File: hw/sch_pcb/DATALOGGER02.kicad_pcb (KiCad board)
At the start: 2 copper layers, 80.8 x 101.1 mm, 90 parts, among them J1 HEADER_2x01_PARALLEL, J10 HEADER_2x03_PARALLEL, J11 HEADER_2x01, J12 HEADER_2x01_PARALLEL, J13 HEADER_2x01_PARALLEL, J14 HEADER_2x01_PARALLEL, J15 HEADER_2x01_PARALLEL, J16 HEADER_2x01_PARALLEL, J17 HEADER_2x01_PARALLEL, J18 HEADER_2x01_PARALLEL, J19 HEADER_2x01_PARALLEL, J2 HEADER_2x01_PARALLEL, J20 HEADER_2x01_PARALLEL, J21 HEADER_2x01, J22 HEADER_2x01_PARALLEL, J23 HEADER_2x01_PARALLEL, J24 HEADER_2x01_PARALLEL, J25 HEADER_2x01_PARALLEL, J26 HEADER_2x01_PARALLEL, J27 HEADER_2x01_PARALLEL, J28 HEADER_2x01_PARALLEL, J29 HEADER_2x01_PARALLEL, J3 HEADER_2x01_PARALLEL, J30 HEADER_2x01_PARALLEL, J31 HEADER_2x03, J32 HEADER_2x01, J33 HEADER_2x03_PARALLEL, J34 MCC-SD (kouka z modulu), J4 HEADER_2x01_PARALLEL, J5 HEADER_2x01_PARALLEL, J6 HEADER_2x03_PARALLEL, J7 MCC-SD, J8 HEADER_2x01_PARALLEL, J9 HEADER_2x01, M2 HOLE, M3 HOLE, M4 HOLE, SW1 5MS1S102AM6QE, U1 ISL21080CIH320Z-TK, U2 TPS22965-Q1, U3 ATMEGA1284P-AU, U4 PCF85263A, U5 LM4041CIM3-1.2(neosazovat), U6 AT24CS64-SSHM, Y1 16MHz, Y2 ABS07-120-32.768KHZ-T

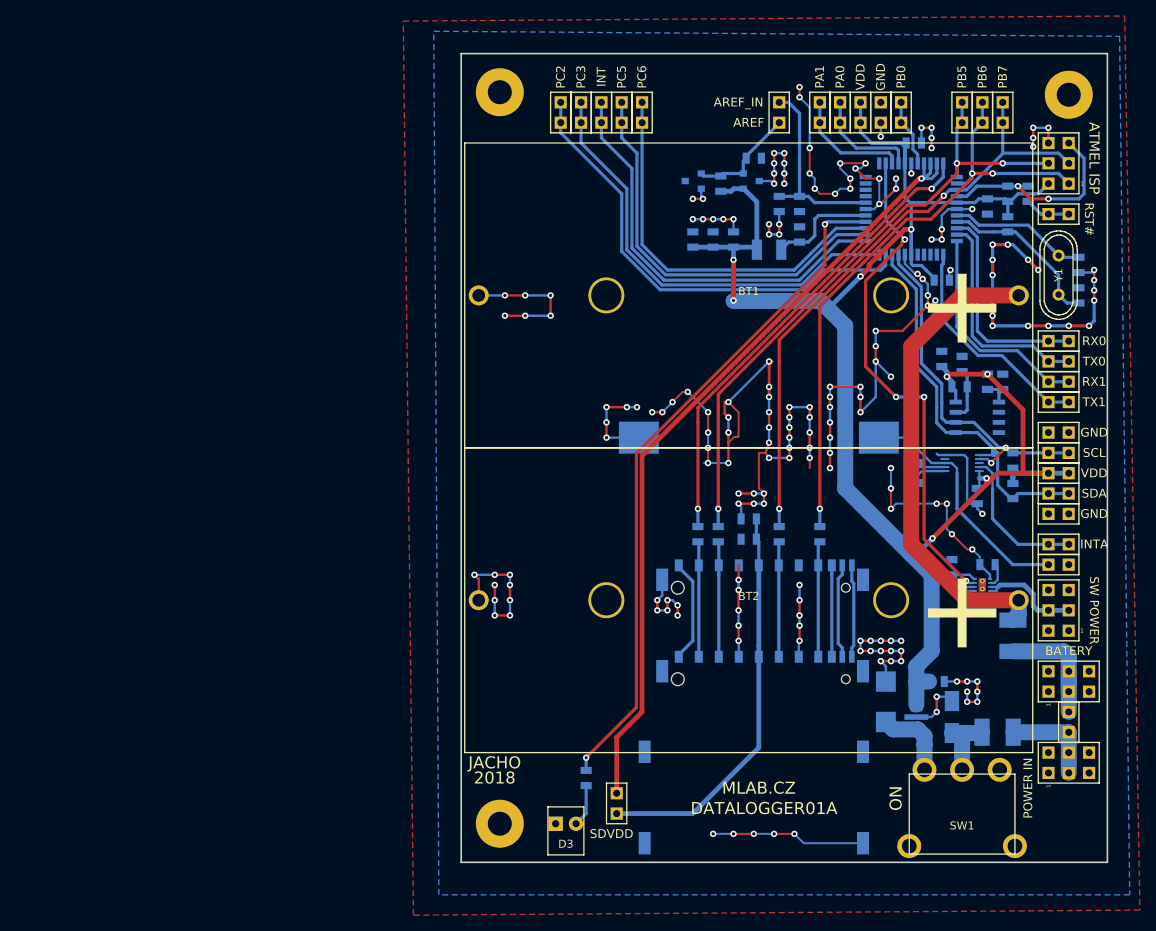
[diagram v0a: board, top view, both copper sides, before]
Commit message: progress?
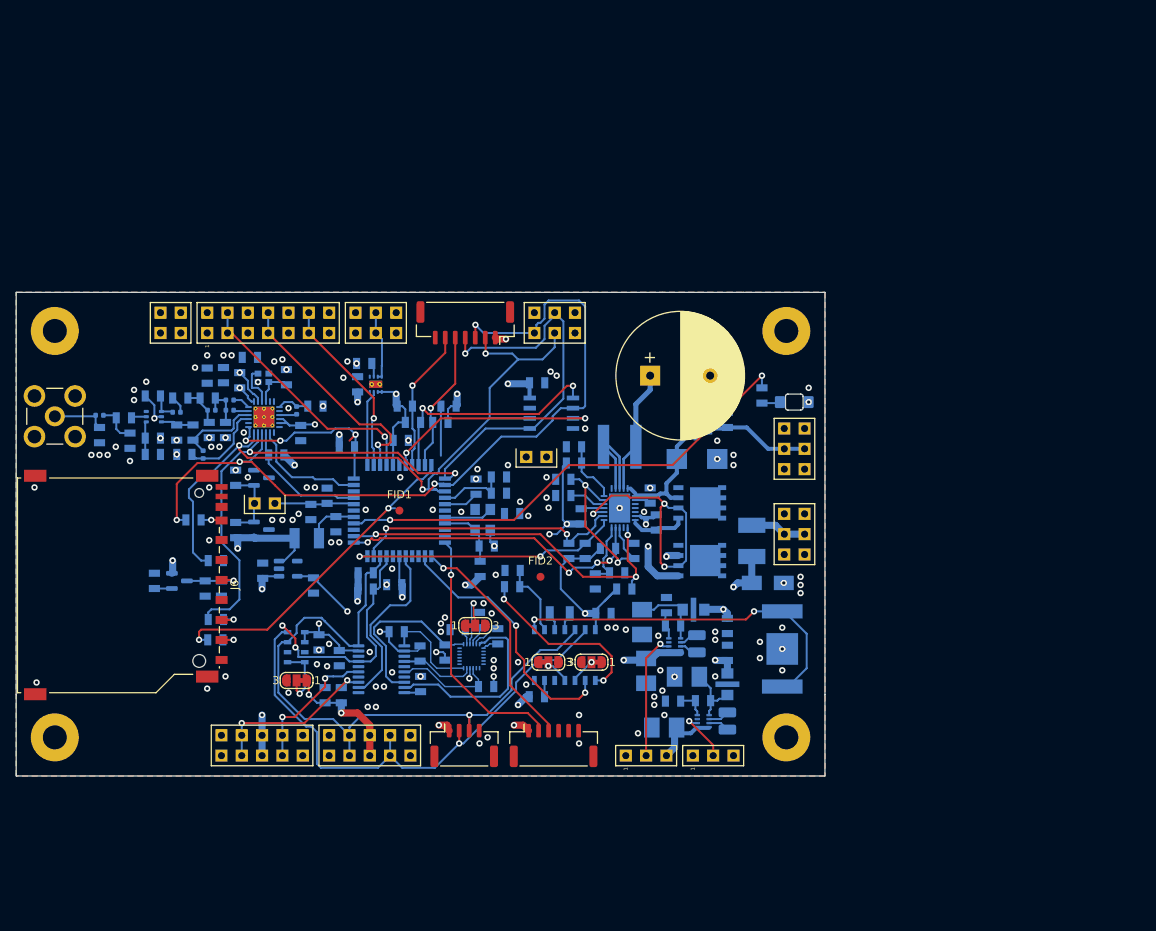
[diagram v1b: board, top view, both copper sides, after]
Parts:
- removed BT2: BX0037, Mlab_Batery:BX0037
- removed BT3: Battery_Cell-device, Mlab_Batery:CH28-2032
- removed C11: 10uF, Mlab_R:SMD-0805
- removed C12: 1nF, Mlab_R:SMD-0805
- removed C13: 100nF, Mlab_R:SMD-0805
- removed D3: HLMP-K150+FIX-LED-313, Mlab_D:FIX-LED-313
- removed F2: 750mA, Mlab_F:1812
- removed J14, J15, J16, J17, J18, J22, J25, J26, J27, J28, J29, J30: HEADER_2x01_PARALLEL, Mlab_Pin_Headers:Straight_2x01
- removed J21, J32: HEADER_2x01, Mlab_Pin_Headers:Straight_2x01
- removed J31: HEADER_2x03, Mlab_Pin_Headers:Straight_2x03
- removed J33: HEADER_2x03_PARALLEL, Mlab_Pin_Headers:Straight_2x03
- removed J34: MCC-SD (kouka z modulu), Mlab_CON:MCC-SD
- removed M2, M3, M4: HOLE, Mlab_Mechanical:MountingHole_3mm
- removed R12: 0R, Mlab_R:SMD-0805
- removed R4: 100, Mlab_R:SMD-0805
- removed R7: 10k, Mlab_R:SMD-0805
- removed SW1: 5MS1S102AM6QE, Mlab_SW:5MS1S102AM6QE
- removed Y1: 16MHz, Mlab_XTAL:Crystal_HC49-U_Vertical
- added C23: 10uF, Mlab_C:SMD-0805, B.Cu at (74.7, 113.5)
- added C24: 100nF, Mlab_C:SMD-0805, B.Cu at (124.5, 116.6)
- added C25: 100nF, Mlab_C:SMD-0805, B.Cu at (76.7, 113.5)
- added C26: 1nF, Mlab_C:SMD-0805, B.Cu at (119.4, 101.9)
- added C27: 1uF, Mlab_C:SMD-0805, B.Cu at (81.9, 111.3)
- added C28: 50F, Mlab_C:C_Radial_D16_L25_P7.5, F.Cu at (130.3, 86.9)
- added C29: 100uF, Mlab_C:TantalC_SizeC_Reflow, B.Cu at (136.2, 97.3)
- added C30: EMI_Filter_C, Mlab_L:FIR_0805, B.Cu at (136.1, 93.5)
- added C31: 1uF, Mlab_C:SMD-0805, B.Cu at (88.2, 113.1)
- added C32: 100nF, Mlab_C:SMD-0805, B.Cu at (140.0, 92.4)
- added C33: 47uF, Mlab_C:TantalC_SizeB_Reflow, B.Cu at (134.9, 124.5)
- added C34: 47uF, Mlab_C:TantalC_SizeB_Reflow, B.Cu at (129.3, 117.7)
- added C35: EMI_Filter_C, Mlab_L:FIR_0805, B.Cu at (140.0, 125.4)
- added C36: EMI_Filter_C, Mlab_L:FIR_0805, B.Cu at (135.7, 116.1)
- added C37: 100nF, Mlab_C:SMD-0805, B.Cu at (140.0, 121.5)
- added C38: 100nF, Mlab_C:SMD-0805, B.Cu at (140.0, 118.2)
- added C39: 22uF, Mlab_C:TantalC_SizeB_Reflow, B.Cu at (129.8, 123.8)
- added C40: 22uF, Mlab_C:TantalC_SizeB_Reflow, B.Cu at (132.1, 130.9)
- added C41: -, Mlab_C:SMD-0805, B.Cu at (80.3, 84.6)
- added C42: -, Mlab_C:SMD-0805, B.Cu at (84.8, 87.1)
- added C43: 470nF, Mlab_C:SMD-0805, B.Cu at (88.5, 90.7)
- added C44: 1uF, Mlab_C:SMD-0805, B.Cu at (86.6, 94.0)
- added C45: 100nF, Mlab_C:SMD-0805, B.Cu at (79.0, 87.4)
- added C46: 47nF, Mlab_C:SMD-0805, B.Cu at (74.9, 86.9)
- added C47: 1p8, Mlab_C:SMD-0805, B.Cu at (72.1, 96.7)
- added C48: 47pF, Mlab_C:SMD-0805, B.Cu at (77.0, 86.8)
- added C49: 2p4, Mlab_C:SMD-0805, B.Cu at (73.2, 94.0)
- added C50: -, Mlab_C:SMD-0805, B.Cu at (77.2, 93.7)
- added C51: -, Mlab_C:SMD-0805, B.Cu at (71.1, 94.0)
- added C52: 3p3, Mlab_C:SMD-0805, B.Cu at (75.0, 89.7)
- added C53: 5p6, Mlab_C:SMD-0805, B.Cu at (75.2, 93.7)
- added C54: 39pF, Mlab_C:SMD-0805, B.Cu at (71.6, 89.7)
- added C55: 2p2, Mlab_C:SMD-0805, B.Cu at (68.1, 89.4)
- added C56: 1nF, Mlab_C:SMD-0805, B.Cu at (68.1, 94.7)
- added C57: 39pF, Mlab_C:SMD-0805, B.Cu at (64.5, 92.1)
- added C58: 3p3, Mlab_C:SMD-0805, B.Cu at (65.3, 95.0)
- added C59: 3p3, Mlab_C:SMD-0805, B.Cu at (61.5, 94.3)
- added D1: HLMP-K150+FIX-LED-313, Mlab_D:LED_1206_mill, B.Cu at (148.3, 90.2)
- added FID1: Fiducial, Fiducial:Fiducial_1mm_Mask2mm, F.Cu at (98.9, 103.7)
- added FID2: Fiducial, Fiducial:Fiducial_1mm_Mask2mm, F.Cu at (116.6, 112.0)
- added H1: MountingHole_Pad, Mlab_Mechanical:MountingHole_3mm, F.Cu at (55.9, 132.1)
- added H2: MountingHole_Pad, Mlab_Mechanical:MountingHole_3mm, F.Cu at (147.3, 132.1)
- added H3: MountingHole_Pad, Mlab_Mechanical:MountingHole_3mm, F.Cu at (147.3, 81.3)
- added H4: MountingHole_Pad, Mlab_Mechanical:MountingHole_3mm, F.Cu at (55.9, 81.3)
- added IC1: CY15B108QN-40SXI, Mlab_IO:SOIC-8_3.9x4.9mm_Pitch1.27mm, B.Cu at (118.0, 91.6)
- added IC2: FM3164-G, Mlab_IO:SOIC-14, B.Cu at (119.6, 121.7)
- added IC3: LTC4041EUFD#PBF, Package_DFN_QFN:QFN-24-1EP_4x5mm_P0.5mm_EP2.65x3.65mm, B.Cu at (126.5, 103.4)
- added JP1: SolderJumper_3_Bridged12, Jumper:SolderJumper-3_P1.3mm_Bridged12_RoundedPad1.0x1.5mm_NumberLabels, F.Cu at (123.0, 122.7)
- added JP2: SolderJumper_3_Bridged12, Jumper:SolderJumper-3_P1.3mm_Bridged12_RoundedPad1.0x1.5mm_NumberLabels, F.Cu at (117.6, 122.7)
- added JP3: SolderJumper_3_Bridged12, Jumper:SolderJumper-3_P1.3mm_Bridged12_RoundedPad1.0x1.5mm_NumberLabels, F.Cu at (86.1, 125.0)
- added JP4: SolderJumper_3_Bridged12, Jumper:SolderJumper-3_P1.3mm_Bridged12_RoundedPad1.0x1.5mm_NumberLabels, F.Cu at (108.4, 118.1)
- added L10: 4n7, Inductor_SMD:L_0402_1005Metric, B.Cu at (71.1, 91.4)
- added L11: 9n1, Inductor_SMD:L_0402_1005Metric, B.Cu at (61.5, 91.8)
- added L2: XAL-6030-182 1.8 uH, XAL6030181MEC:XAL6030181MEC, B.Cu at (126.5, 95.8)
- added L3: 1uH - DFE252012P-1R0M=P2, Inductor_SMD:L_1008_2520Metric, B.Cu at (140.0, 130.0)
- added L4: 1uH - DFE252012P-1R0M=P2, Inductor_SMD:L_1008_2520Metric, B.Cu at (136.1, 120.4)
- added L5: 15uH, Inductor_SMD:L_0402_1005Metric, B.Cu at (86.1, 91.2)
- added L6: 15nH, Inductor_SMD:L_0402_1005Metric, B.Cu at (74.4, 96.7)
- added L7: 0R, Inductor_SMD:L_0402_1005Metric, B.Cu at (77.7, 91.2)
- added L8: 47nH, Inductor_SMD:L_0402_1005Metric, B.Cu at (77.7, 89.9)
- added L9: 2n5, Inductor_SMD:L_0402_1005Metric, B.Cu at (75.5, 91.2)
- added Q1: DMP2045UQ-7, Package_TO_SOT_SMD:SOT-23, B.Cu at (71.5, 112.5)
- added Q2: SIR424DP, SIR424DP:SIR106DPT1RE3, B.Cu at (136.6, 110.0)
- added Q3: SIR424DP, SIR424DP:SIR106DPT1RE3, B.Cu at (136.6, 102.8)
- added R14: 10k, Mlab_R:SMD-0805, B.Cu at (98.6, 118.9)
- added R17: 10k, Mlab_R:SMD-0805, B.Cu at (104.6, 121.5)
- added R18: 10k, Mlab_R:SMD-0805, B.Cu at (89.7, 126.8)
- added R19: 10k, Mlab_R:SMD-0805, B.Cu at (91.7, 126.8)
- added R20: 470R, Mlab_R:SMD-0805, B.Cu at (68.3, 112.5)
- added R21: 10k, Mlab_R:SMD-0805, B.Cu at (116.1, 127.0)
- added R22: 150k, Mlab_R:SMD-0805, B.Cu at (113.0, 113.2)
- added R23: 56k, Mlab_R:SMD-0805, B.Cu at (113.1, 111.2)
- added R24: 100, Mlab_R:SMD-0805, B.Cu at (75.9, 119.9)
- added R25: 100, Mlab_R:SMD-0805, B.Cu at (76.0, 117.3)
- added R26: 100, Mlab_R:SMD-0805, B.Cu at (76.0, 110.0)
- added R27: 100, Mlab_R:SMD-0805, B.Cu at (73.2, 104.9)
- added R28: 2k2, Mlab_R:SMD-0805, B.Cu at (144.3, 89.3)
- added R29: 150k, Mlab_R:SMD-0805, B.Cu at (120.8, 97.8)
- added R30: 56k, Mlab_R:SMD-0805, B.Cu at (120.8, 95.8)
- added R31: 1M, Mlab_R:SMD-0805, B.Cu at (127.1, 113.5)
- added R32: 100k, Mlab_R:SMD-0805, B.Cu at (125.0, 108.5)
- added R33: 100k, Mlab_R:SMD-0805, B.Cu at (122.2, 108.8)
- added R34: 100k, Mlab_R:SMD-0805, B.Cu at (120.1, 108.8)
- added R35: 6.2k 1/8W, Mlab_R:SMD-0805, B.Cu at (121.7, 104.5)
- added R36: 2k, Mlab_R:SMD-0805, B.Cu at (130.3, 101.9)
- added R37: 25mR, Mlab_R:SMD-0805, B.Cu at (131.1, 105.2)
- added R38: 523k (E96), Mlab_R:SMD-0805, B.Cu at (128.3, 108.8)
- added R39: 100k, Mlab_R:SMD-0805, B.Cu at (119.4, 99.8)
- added R40: 220k, Mlab_R:SMD-0805, B.Cu at (126.2, 111.5)
- added R41: 100k, Mlab_R:SMD-0805, B.Cu at (123.4, 112.6)
- added R42: 806k, Mlab_R:SMD-0805, B.Cu at (136.9, 127.5)
- added R43: 91k, Mlab_R:SMD-0805, B.Cu at (133.2, 127.6)
- added R44: 511k, Mlab_R:SMD-0805, B.Cu at (133.2, 118.2)
- added R45: 91k, Mlab_R:SMD-0805, B.Cu at (132.3, 115.5)
- added R46: 10k, Mlab_R:SMD-0805, B.Cu at (83.6, 96.8)
- added R47: 100R, Mlab_R:SMD-0805, B.Cu at (68.1, 96.7)
- added R48: 10k, Mlab_R:SMD-0805, B.Cu at (92.4, 95.8)
- added U10: TPS631000DRLR, Package_TO_SOT_SMD:SOT-583-8, B.Cu at (133.4, 120.5)
- added U11: SX1262, Package_DFN_QFN:QFN-24-1EP_4x4mm_P0.5mm_EP2.6x2.6mm_ThermalVias, B.Cu at (82.0, 92.0)
- added U12: PE4259, Package_TO_SOT_SMD:SOT-363_SC-70-6, B.Cu at (68.3, 92.0)
- added U7: MS5611-01BA, Package_LGA:LGA-8_3x5mm_P1.25mm, B.Cu at (86.0, 120.8)
- added U8: MIC5504-1.8YM5-TR, Package_TO_SOT_SMD:SOT-23-5, B.Cu at (85.0, 111.0)
- added U9: TPS631000DRLR, Package_TO_SOT_SMD:SOT-583-8, B.Cu at (136.9, 130.0)
- added Y3: 32MHz, Mlab_XTAL:Crystal_SMD_NX2016SA, B.Cu at (82.0, 87.1)
- added Y6: 8MHz LFXTAL083138, Mlab_XTAL:Crystal SMD CFPX-180, B.Cu at (109.4, 104.9)
- BT1: value BX0037 -> Battery_Cell-device 3V; footprint Mlab_Batery:BX0037 -> Battery:BatteryHolder_Keystone_2998_1x6.8mm; moved to B.Cu
- C1, C15, C17, C18, C19, C2, C22, C5, C6: footprint Mlab_R:SMD-0805 -> Mlab_C:SMD-0805
- C10: value EMI_Filter_C -> 100nF; footprint Mlab_L:FIR1 -> Mlab_C:SMD-0805
- C14: value 10uF -> 100nF; footprint Mlab_R:SMD-0805 -> Mlab_C:SMD-0805
- C16: value 4u7 -> 100nF; footprint Mlab_R:SMD-0805 -> Mlab_C:SMD-0805
- C20: value 100nF -> 1uF; footprint Mlab_R:SMD-0805 -> Mlab_C:SMD-0805
- C21: value 100nF -> 1nF; footprint Mlab_R:SMD-0805 -> Mlab_C:SMD-0805
- C3, C4: value 100nF -> 15pF; footprint Mlab_R:SMD-0805 -> Mlab_C:SMD-0805
- C7: value 1uF -> 10uF; footprint Mlab_R:SMD-0805 -> Mlab_C:SMD-0805
- C8: value 100nF -> 4u7; footprint Mlab_R:SMD-0805 -> Mlab_C:SMD-0805
- C9: value 47uF -> 100nF; footprint Mlab_C:TantalC_SizeC_Reflow -> Mlab_C:SMD-0805
- D2: footprint Mlab_D:SMA_Standard -> Mlab_D:Diode-SMA_Standard
- F1: value 750mA -> 1.2A
- J10: value HEADER_2x03_PARALLEL -> HEADER_2x05_PARALLEL; footprint Mlab_Pin_Headers:Straight_2x03 -> Mlab_Pin_Headers:Straight_2x05
- J11: value HEADER_2x01 -> HEADER_2x07_PARALLEL; footprint Mlab_Pin_Headers:Straight_2x01 -> Mlab_Pin_Headers:Straight_2x07
- J12: value HEADER_2x01_PARALLEL -> HEADER_2x05_PARALLEL; footprint Mlab_Pin_Headers:Straight_2x01 -> Mlab_Pin_Headers:Straight_2x05
- J13: value HEADER_2x01_PARALLEL -> HEADER_2x02_PARALLEL; footprint Mlab_Pin_Headers:Straight_2x01 -> Mlab_Pin_Headers:Straight_2x02
- J19, J20: value HEADER_2x01_PARALLEL -> Conn_01x03_Male; footprint Mlab_Pin_Headers:Straight_2x01 -> Mlab_Pin_Headers:Straight_1x03
- J2: value HEADER_2x01_PARALLEL -> HEADER_2x01
- J23: value HEADER_2x01_PARALLEL -> MCX; footprint Mlab_Pin_Headers:Straight_2x01 -> Mlab_CON:MCX
- J24, J4, J5: value HEADER_2x01_PARALLEL -> HEADER_2x03_PARALLEL; footprint Mlab_Pin_Headers:Straight_2x01 -> Mlab_Pin_Headers:Straight_2x03
- J3: value HEADER_2x01_PARALLEL -> HEADER_2x03; footprint Mlab_Pin_Headers:Straight_2x01 -> Mlab_Pin_Headers:Straight_2x03
- J6: value HEADER_2x03_PARALLEL -> MCC-SD (kouka z modulu); footprint Mlab_Pin_Headers:Straight_2x03 -> Mlab_CON:MCC-SD
- J7: value MCC-SD -> Conn_01x06_Female; footprint Connector_Card:SD_TE_2041021 -> Connector_JST:JST_GH_SM06B-GHS-TB_1x06-1MP_P1.25mm_Horizontal; moved to F.Cu
- J8: value HEADER_2x01_PARALLEL -> Conn_01x07_Female; footprint Mlab_Pin_Headers:Straight_2x01 -> Connector_JST:JST_GH_SM07B-GHS-TB_1x07-1MP_P1.25mm_Horizontal
- J9: value HEADER_2x01 -> Conn_01x04_Female; footprint Mlab_Pin_Headers:Straight_2x01 -> Connector_JST:JST_GH_SM04B-GHS-TB_1x04-1MP_P1.25mm_Horizontal
- R1: value 100 -> -
- R10: value 2k2 -> 10k
- R11, R16, R8: value - -> 10k
- R15: value 0R -> 10k
- R2: value 100 -> 4k7
- R3: value 100 -> 10k
- R5: value 4k7 -> 10k
- U2: value TPS22965-Q1 -> LM4041CIM3-1.2(neosazovat); footprint Package_SON:WSON-8-1EP_2x2mm_P0.5mm_EP0.9x1.6mm_ThermalVias -> Package_TO_SOT_SMD:SOT-23
- U4: value PCF85263A -> TXS0108EPW; footprint Mlab_IO:TSSOP-10_3x3mm_Pitch0.5mm -> Package_SO:TSSOP-20_4.4x6.5mm_P0.65mm
- U5: value LM4041CIM3-1.2(neosazovat) -> ICM-20948; footprint Package_TO_SOT_SMD:SOT-23 -> Sensor_Motion:InvenSense_QFN-24_3x3mm_P0.4mm
- U6: value AT24CS64-SSHM -> TPS22965-Q1; footprint Package_SO:SOIC-8_3.9x4.9mm_P1.27mm -> Package_SON:WSON-8-1EP_2x2mm_P0.5mm_EP0.9x1.6mm_ThermalVias
- Y2: value ABS07-120-32.768KHZ-T -> 6pF crystal - 32.768kHz
- moved J6 118.5 mm to (64.8, 113.0), turned to -90 degrees
- moved C5 108.7 mm to (78.5, 99.6), turned to 90 degrees
- moved C16 103.8 mm to (91.4, 122.2)
- moved J23 102.9 mm to (55.9, 91.9), turned to 0 degrees
- moved J2 99.4 mm to (82.1, 102.8), turned to 0 degrees
- moved U2 91.1 mm to (81.7, 99.6)
- moved J9 88.4 mm to (107.1, 133.1), turned to 0 degrees
- moved J4 88.0 mm to (96.0, 80.3), turned to 90 degrees
- moved J10 87.7 mm to (95.2, 133.1), turned to -90 degrees
- moved J12 87.5 mm to (81.8, 133.1)
- moved C22 85.5 mm to (88.9, 120.2), turned to -90 degrees
- moved R11 81.3 mm to (94.7, 111.5), turned to 0 degrees
- moved C19 80.6 mm to (109.0, 117.4), turned to 90 degrees
- moved C7 80.4 mm to (87.9, 103.9), turned to -90 degrees
- moved C21 80.3 mm to (94.6, 85.3), turned to 180 degrees
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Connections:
- net Net-(D2-Pad1) renamed UNREG_POWER_INPUT
- C1 pad 1: VDD -> +3.3V
- C10 pad 1: Net-(C10-Pad1) -> /Microcontroller/AVCC
- C14 pad 1: Net-(C14-Pad1) -> GND
- C14 pad 2: GND -> +1V8
- C15 pad 1: /SD_VDD -> +1V8
- C16 pad 1: /RST#_P -> +3.3V
- C16 pad 2: /RST# -> GND
- C17 pad 1: Net-(C14-Pad1) -> +3.3V
- C18 pad 1: VDD -> +3.3V
- C19 pad 1: VDD -> Net-(U5-REGOUT)
- C2 pad 1: VDD -> +3.3V
- C20 pad 1: VDD -> +3.3V
- C21 pad 1: VDD -> Net-(U6-CT)
- C22 pad 1: VDD -> +3.3V
- C3 pad 1: VDD -> GND
- C3 pad 2: GND -> Net-(U3-XTAL2)
- C4 pad 1: /AREF -> GND
- C4 pad 2: GND -> Net-(U3-XTAL1)
- C5 pad 1: Net-(C5-Pad1) -> /Microcontroller/AREF
- C6 pad 1: /AVCC -> +3.3V
- C7 pad 1: VDD -> Net-(U3-AREF)
- C8 pad 1: Net-(C8-Pad1) -> /Microcontroller/RST#_P
- C8 pad 2: GND -> /Microcontroller/RST#
- C9 pad 1: Net-(C10-Pad1) -> Net-(U3-AREF)
- J1 pad 1: GND -> /Microcontroller/RST#
- J1 pad 2: GND -> /Microcontroller/RST#
- J10 pad 3: Net-(J10-Pad3) -> SCL_I2C
- J10 pad 4: Net-(J10-Pad3) -> SCL_I2C
- J10 pad 5: GND -> +3.3V
- J10 pad 6: GND -> +3.3V
- J11 pad 1: Net-(J11-Pad1) -> GND
- J11 pad 2: /SD_VDD -> GND
- J12 pad 1: /PC2 -> GND
- J12 pad 2: /PC2 -> GND
- J13 pad 1: /PC3 -> /Telemetry/DIO3
- J13 pad 2: /PC3 -> /Telemetry/DIO3
- J19 pad 1: /RX1 -> GND
- J19 pad 2: /RX1 -> Net-(J19-Pin_2)
- J2 pad 1: /PC0 -> /Microcontroller/AREF
- J2 pad 2: /PC0 -> Net-(U3-AREF)
- J20 pad 1: /TX1 -> GND
- J20 pad 2: /TX1 -> Net-(J20-Pin_2)
- J23 pad 1: /PA1 -> Net-(C59-Pad2)
- J23 pad 2: /PA1 -> GND
- J24 pad 1: VDD -> GND
- J24 pad 2: VDD -> GND
- J3 pad 1: VDD -> MISO_SPI
- J3 pad 2: VDD -> +3.3V
- J4 pad 1: /PC1 -> GND
- J4 pad 2: /PC1 -> GND
- J6 pad 1: GND -> Net-(J6-CD/DAT3)
- J6 pad 2: GND -> Net-(J6-CMD)
- J6 pad 3: Net-(F2-Pad1) -> GND
- J6 pad 4: Net-(F2-Pad1) -> /Peripherals/sd_card_power
- J6 pad 5: GND -> Net-(J6-CLK)
- J7 pad 1: Net-(J34-Pad1) -> +5V
- J7 pad 2: Net-(J34-Pad2) -> RX1
- J7 pad 3: GND -> TX1
- J7 pad 4: /SD_VDD -> unconnected-(J7-Pin_4-Pad4)
- J7 pad 5: Net-(J34-Pad5) -> unconnected-(J7-Pin_5-Pad5)
- J8 pad 1: /RST# -> +5V
- J8 pad 2: /RST# -> SCK_SPI
- J9 pad 1: /AREF -> +5V
- J9 pad 2: Net-(C14-Pad1) -> SCL_I2C
- L1 pad 1: VDD -> +3.3V
- L1 pad 2: /AVCC -> /Microcontroller/AVCC
- R1 pad 1: Net-(J34-Pad1) -> Net-(U3-XTAL1)
- R1 pad 2: /PB4 -> +3.3V
- R10 pad 1: Net-(D3-Pad2) -> +3.3V
- R10 pad 2: /LED -> SCL_I2C
- R11 pad 1: VDD -> +3.3V
- R11 pad 2: Net-(R11-Pad2) -> SDA_I2C
- R15 pad 1: GND -> +1V8
- R15 pad 2: Net-(R15-Pad2) -> /Peripherals/SCL_I2C_1V8
- R16 pad 1: Net-(R15-Pad2) -> +1V8
- R16 pad 2: VDD -> /Peripherals/AUX_SDA_1V8
- R2 pad 1: Net-(J34-Pad2) -> /Microcontroller/AREF
- R2 pad 2: /PB5 -> +3.3V
- R3 pad 1: Net-(J34-Pad5) -> /Microcontroller/RST#_P
- R3 pad 2: /PB7 -> +3.3V
- R5 pad 1: /AREF -> +3.3V
- R5 pad 2: VDD -> CS_CONN_1
- R6 pad 1: /PC1 -> +3.3V
- R6 pad 2: VDD -> CS_FRAM
- R8 pad 1: VDD -> +3.3V
- R8 pad 2: Net-(C8-Pad1) -> CS_CONN_2
- R9 pad 1: /RST#_P -> +3.3V
- R9 pad 2: VDD -> CS_SDCARD
- U1 pad 1: VDD -> +3.3V
- U1 pad 2: /AREF -> /Microcontroller/AREF
- U2 pad 1: VDD -> /Microcontroller/AREF
- U2 pad 2: VDD -> GND
- U2 pad 3: /PA2 -> (no net)
- U3 pad 1: /PB5 -> MOSI_SPI
- U3 pad 10: /TX0 -> TX0
- U3 pad 11: /RX1 -> RX1
- U3 pad 12: /TX1 -> TX1
- U3 pad 13: (no net) -> CNT2
- U3 pad 14: (no net) -> unconnected-(U3-(PCINT294/OC1A)PD5-Pad14)
- U3 pad 15: (no net) -> unconnected-(U3-(PCINT30/OC2B/ICP)PD6-Pad15)
- U3 pad 16: (no net) -> INT1
- U3 pad 17: VDD -> +3.3V
- U3 pad 19: /PC0 -> SCL_I2C
- U3 pad 2: /PB6 -> MISO_SPI
- U3 pad 20: /PC1 -> SDA_I2C
- U3 pad 21: /PC2 -> PFO
- U3 pad 22: /PC3 -> CAPGD
- U3 pad 23: /INT -> SYSGD
- U3 pad 24: /PC5 -> CAPFLT
- U3 pad 25: /PC6 -> unconnected-(U3-(PCINT22/TOSC1)PC6-Pad25)
- U3 pad 26: /LED -> LED
- U3 pad 27: /AVCC -> /Microcontroller/AVCC
- U3 pad 29: Net-(C14-Pad1) -> Net-(U3-AREF)
- U3 pad 3: /PB7 -> SCK_SPI
- U3 pad 30: (no net) -> RST_LORA
- U3 pad 31: (no net) -> DIO_LORA
- U3 pad 32: (no net) -> BUSY_LORA
- U3 pad 33: (no net) -> CS_LORA
- U3 pad 34: (no net) -> IO_SWCH
- U3 pad 35: /PA2 -> PA2
- U3 pad 36: /PA1 -> PA1
- U3 pad 37: /PA0 -> PA0
- U3 pad 38: VDD -> +3.3V
- U3 pad 4: /RST#_P -> /Microcontroller/RST#_P
- U3 pad 40: /PB0 -> WP_FRAM
- U3 pad 41: Net-(J11-Pad1) -> CS_CONN_1
- U3 pad 42: Net-(J11-Pad1) -> CS_FRAM
- U3 pad 43: Net-(J11-Pad1) -> CS_CONN_2
- U3 pad 44: /PB4 -> CS_SDCARD
- U3 pad 5: VDD -> +3.3V
- U3 pad 7: Net-(C5-Pad1) -> Net-(U3-XTAL2)
- U3 pad 8: Net-(C8-Pad1) -> Net-(U3-XTAL1)
- U3 pad 9: /RX0 -> RX0
- U4 pad 1: Net-(U4-Pad1) -> /Peripherals/SDA_I2C_1V8
- U4 pad 10: VDD -> +1V8
- U4 pad 2: Net-(U4-Pad2) -> +1V8
- U4 pad 3: Net-(BT3-Pad1) -> GND
- U4 pad 4: (no net) -> /Peripherals/SCL_I2C_1V8
- U4 pad 6: /PC1 -> /Peripherals/AUX_SDA_1V8
- U4 pad 7: /PC0 -> GND
- U4 pad 8: (no net) -> /Peripherals/AUX_SCL_1V8
- U4 pad 9: /INTA -> /Peripherals/INT1_1V8
- U5 pad 1: /AREF -> unconnected-(U5-NC-Pad1)
- U5 pad 2: GND -> unconnected-(U5-NC-Pad2)
- U5 pad 3: (no net) -> unconnected-(U5-NC-Pad3)
- U6 pad 1: Net-(R11-Pad2) -> +3.3V
- U6 pad 2: GND -> +3.3V
- U6 pad 3: GND -> IO_SWCH
- U6 pad 4: GND -> +3.3V
- U6 pad 5: /PC1 -> GND
- U6 pad 6: /PC0 -> Net-(U6-CT)
- U6 pad 7: Net-(R15-Pad2) -> Net-(J4-Pad3)
- U6 pad 8: VDD -> Net-(J4-Pad3)
- Y2 pad 1: Net-(U4-Pad2) -> Net-(IC2-X1)
- Y2 pad 2: Net-(U4-Pad1) -> Net-(IC2-X2)
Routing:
- net GND: track 435.8 -> 14.7 mm, vias 191 -> 39
- net +3.3V: track 0.00 -> 347.2 mm, vias 0 -> 23
- net VDD: track 245.9 -> 0.00 mm, vias 8 -> 0
- net +5V: track 0.00 -> 148.4 mm, vias 0 -> 4
- net MOSI_SPI: track 0.00 -> 105.4 mm, vias 0 -> 3
- net MISO_SPI: track 0.00 -> 102.7 mm, vias 0 -> 4
- net Net-(J11-Pad1): track 100.3 -> 0.00 mm, vias 1 -> 0
- net SCL_I2C: track 0.00 -> 97.5 mm, vias 0 -> 3
- net /Power_management/Vdc: track 0.00 -> 94.9 mm, vias 0 -> 1
- net SCK_SPI: track 0.00 -> 91.8 mm, vias 0 -> 3
- net /LED: track 85.8 -> 0.00 mm, vias 2 -> 0
- net SDA_I2C: track 0.00 -> 84.1 mm, vias 0 -> 1
- net /PB5: track 80.1 -> 0.00 mm, vias 3 -> 0
- net /PB6: track 79.4 -> 0.00 mm, vias 3 -> 0
- net /PB7: track 76.1 -> 0.00 mm, vias 2 -> 0
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- added copper zone on In1.Cu, net GND
- added copper zone on In2.Cu, net GND
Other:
- board size 80.8 x 101.1 mm -> 101.1 x 60.5 mm
- copper layers 2 -> 4
- board text removed: "2018"
- board text removed: "AREF"
- board text removed: "AREF_IN"
- board text removed: "ATMEL ISP"
- board text removed: "BATERY"
- board text removed: "DATALOGGER01A"
- board text removed: "GND"
- board text removed: "INT"
- board text removed: "INTA"
- board text removed: "JACHO"
- board text removed: "MLAB.CZ"
- board text removed: "ON"
- board text removed: "PA0"
- board text removed: "PA1"
- board text removed: "PB0"
- board text removed: "PB5"
- board text removed: "PB6"
- board text removed: "PB7"
- board text removed: "PC2"
- board text removed: "PC3"
- board text removed: "PC5"
- board text removed: "PC6"
- board text removed: "POWER IN"
- board text removed: "RST#"
- board text removed: "RX0"
- board text removed: "RX1"
- board text removed: "SCL"
- board text removed: "SDA"
- board text removed: "SDVDD"
- board text removed: "SW POWER"
- board text removed: "TX0"
- board text removed: "TX1"
- board text removed: "VDD"
